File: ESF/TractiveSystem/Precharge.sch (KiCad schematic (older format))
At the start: 37 parts

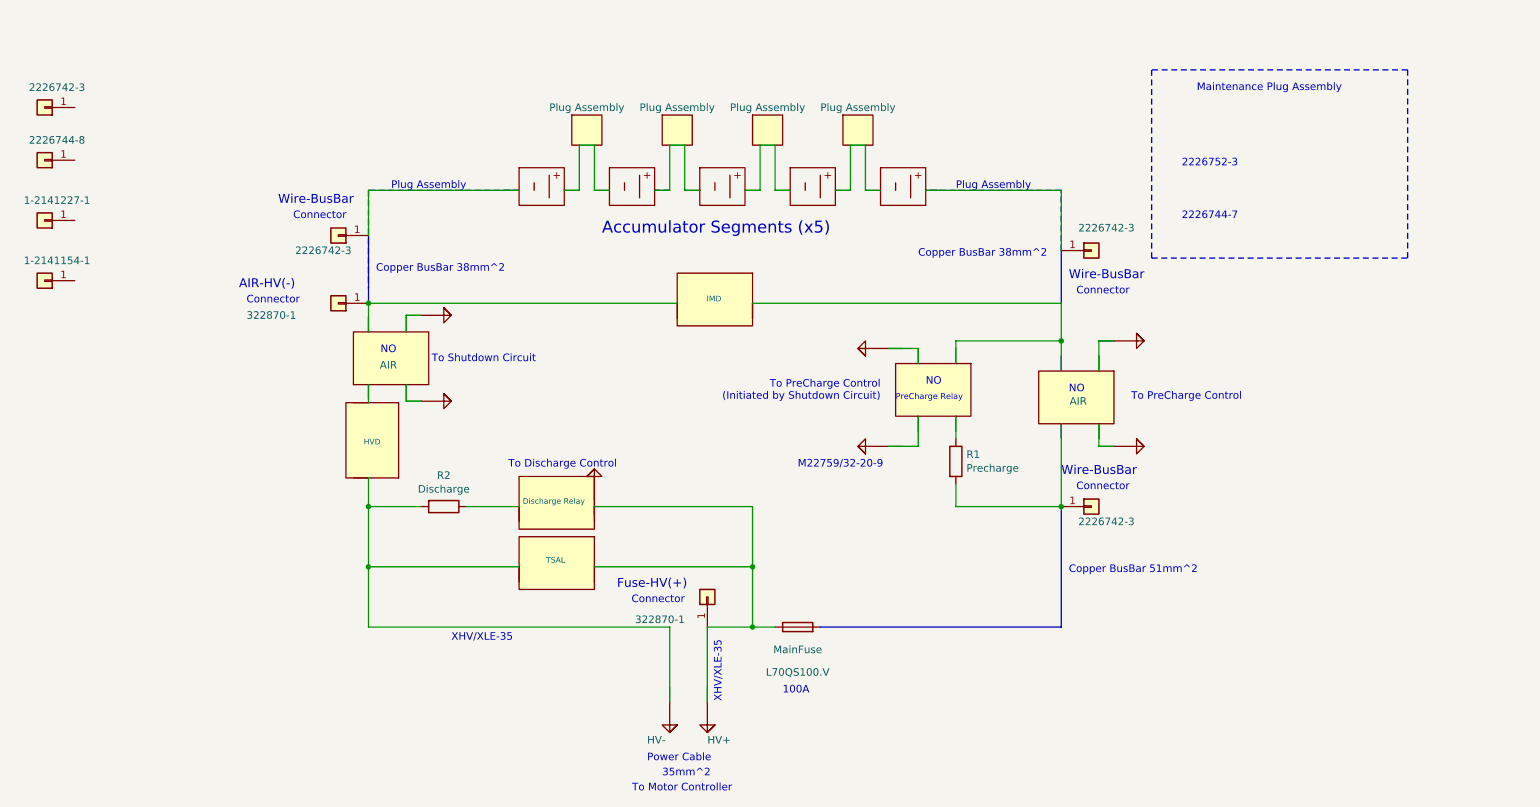
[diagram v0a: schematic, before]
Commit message: Update ESFSymbols.dcm, ESFSymbols.lib, and 3 more files...
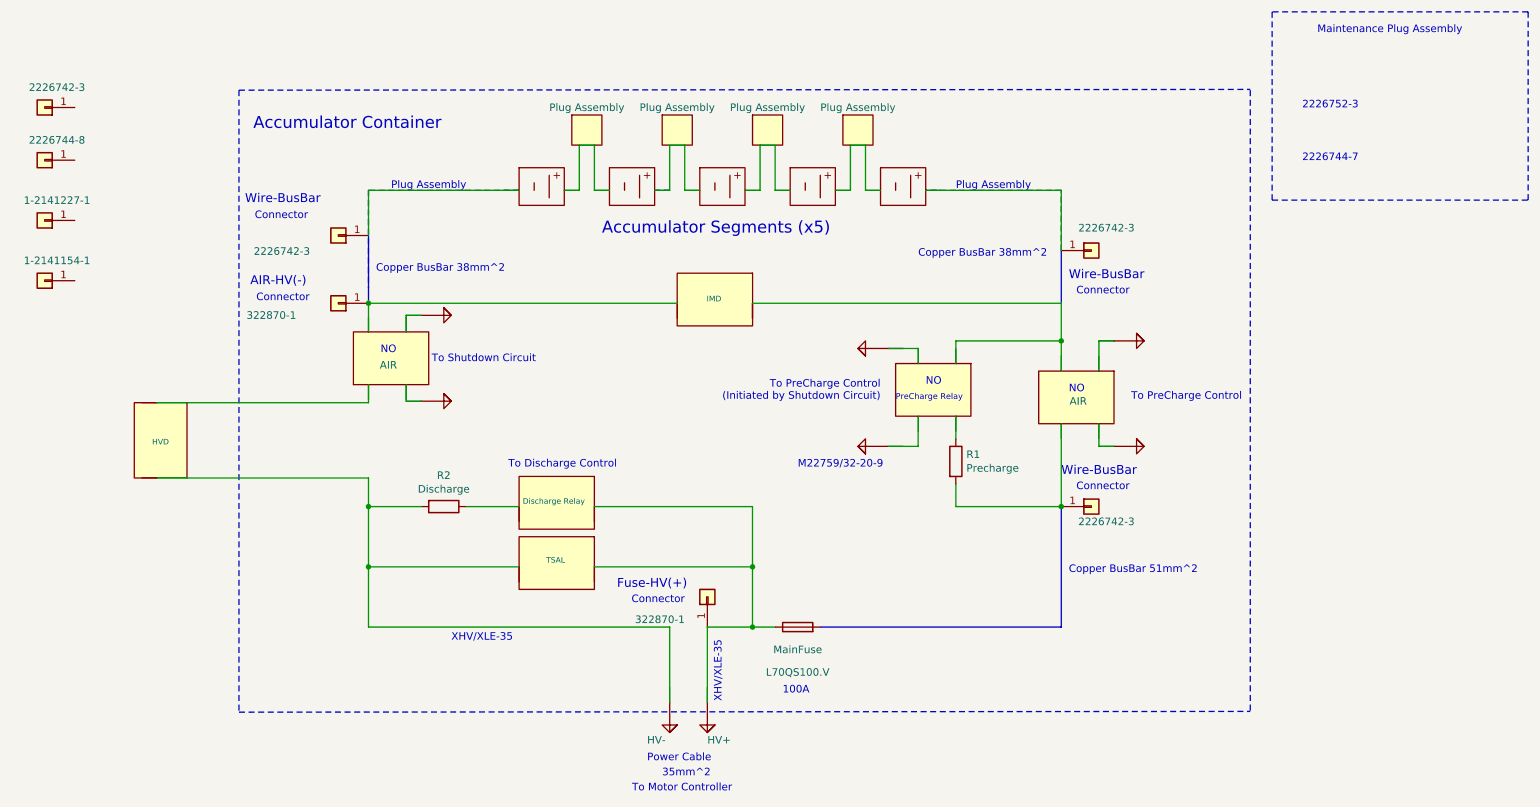
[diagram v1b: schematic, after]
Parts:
- removed U?: HV+, symbol ESFSymbols:HV+
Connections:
- net at V1?.~: now also V?.~; no longer V?.~
- net at V?.~: now also J?.1 (Pin_1); no longer V1?.~
- net at V?.~: now also J?.1 (Pin_1); no longer V?.~
- new net: V1?.~, V?.~
- new net: V?.~, V?.~
- new net: J?.1 (Pin_1), U?.~, U?.~
- new net: U?.~, U?.~, U?.~
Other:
- note added: "Accumulator Container\n"
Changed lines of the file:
@@
 P 3150 2600
 F 0 "J?" H 3068 2375 50  0001 C CNN
-F 1 "2226742-3" H 3250 2700 50  0000 C CNN
+F 1 "2226742-3" H 3525 2705 50  0000 C CNN
 F 2 "" H 3150 2600 50  0001 C CNN
 F 3 "~" H 3150 2600 50  0001 C CNN
@@
 	-1   0    0    1
 $EndComp
-Text Notes 2750 2400 0    59   ~ 0
+Text Notes 2530 2395 0    59   ~ 0
 Wire-BusBar\n
 Text Notes 5000 4950 0    59   ~ 0
 Fuse-HV(+)\n
-Text Notes 2490 2960 0    59   ~ 0
+Text Notes 2565 2940 0    59   ~ 0
 AIR-HV(-)
-Text Notes 2850 2500 0    50   ~ 0
+Text Notes 2595 2500 0    50   ~ 0
 Connector
 Text Notes 5450 5050 2    50   ~ 0
@@
 Text Notes 7050 3600 0    50   ~ 0
 NO
-Text Notes 2540 3060 0    50   ~ 0
+Text Notes 2605 3045 0    50   ~ 0
 Connector
 Wire Wire Line
@@
 Copper BusBar 38mm^2
 $Bitmap
-Pos 9400 2200
+Pos 10200 1815
 Scale 0.400000
 Data
@@
 EndData
 $EndBitmap
-Text Notes 8850 1650 0    50   ~ 0
+Text Notes 9650 1265 0    50   ~ 0
 Maintenance Plug Assembly
 Wire Notes Line style solid rgb(194, 4, 0)
-	8550 2750 10250 2750
+	9350 2365 11050 2365
 Wire Notes Line style solid rgb(194, 0, 18)
-	10250 2750 10250 1500
+	11050 2365 11050 1115
 Wire Notes Line style solid rgb(194, 15, 6)
-	10250 1500 8550 1500
+	11050 1115 9350 1115
 Wire Notes Line style solid rgb(194, 3, 7)
-	8550 1500 8550 2750
+	9350 1115 9350 2365
 Wire Notes Line style solid rgb(194, 13, 6)
 	7950 2700 7950 2300
@@
 Text Notes 7950 4200 0    59   ~ 0
 Wire-BusBar\n
-Text Notes 8750 2500 0    50   ~ 0
+Text Notes 9550 2115 0    50   ~ 0
 2226744-7
-Text Notes 8750 2150 0    50   ~ 0
+Text Notes 9550 1765 0    50   ~ 0
 2226752-3
 Wire Wire Line
@@
 L ESFSymbols:BlackBoxModel_NOConnection U?
 U 1 1 62562F1C
-P 3350 4010
-F 0 "U?" H 3528 4006 50  0001 L CNN
-F 1 "HVD" H 3270 3970 37  0000 L CNN
-F 2 "" H 3350 4010 50  0001 C CNN
-F 3 "" H 3350 4010 50  0001 C CNN
-	1    3350 4010
+P 1945 4010
+F 0 "U?" H 2123 4006 50  0001 L CNN
+F 1 "HVD" H 1865 3970 37  0000 L CNN
+F 2 "" H 1945 4010 50  0001 C CNN
+F 3 "" H 1945 4010 50  0001 C CNN
+	1    1945 4010
 	-1   0    0    1
 $EndComp
@@
 Text Notes 5000 4150 2    50   ~ 0
 To Discharge Control
-$Comp
-L ESFSymbols:HV+ U?
-U 1 1 625638F8
-P 4850 4300
-F 0 "U?" H 4850 4400 50  0001 C CNN
-F 1 "HV+" H 4950 4300 50  0001 L CNN
-F 2 "" H 4850 4300 50  0001 C CNN
-F 3 "" H 4850 4300 50  0001 C CNN
-	1    4850 4300
-	-1   0    0    1
-$EndComp
+Wire Wire Line
+	3350 3710 1945 3710
+Wire Wire Line
+	3350 4210 1945 4210
+Wire Notes Line
+	2490 1635 2490 5765
+Wire Notes Line
+	2490 5765 9205 5760
+Wire Notes Line
+	2490 1635 9205 1630
+Wire Notes Line
+	9205 1635 9205 5765
+Text Notes 2585 1905 0    79   ~ 0
+Accumulator Container\n
 $EndSCHEMATC
